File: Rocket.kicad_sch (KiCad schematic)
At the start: 6 parts, among them U1 BMP280, U2 MPU-6050, U3 ArduinoMicroSD, U4 NEO_6M, U5 FT232RL

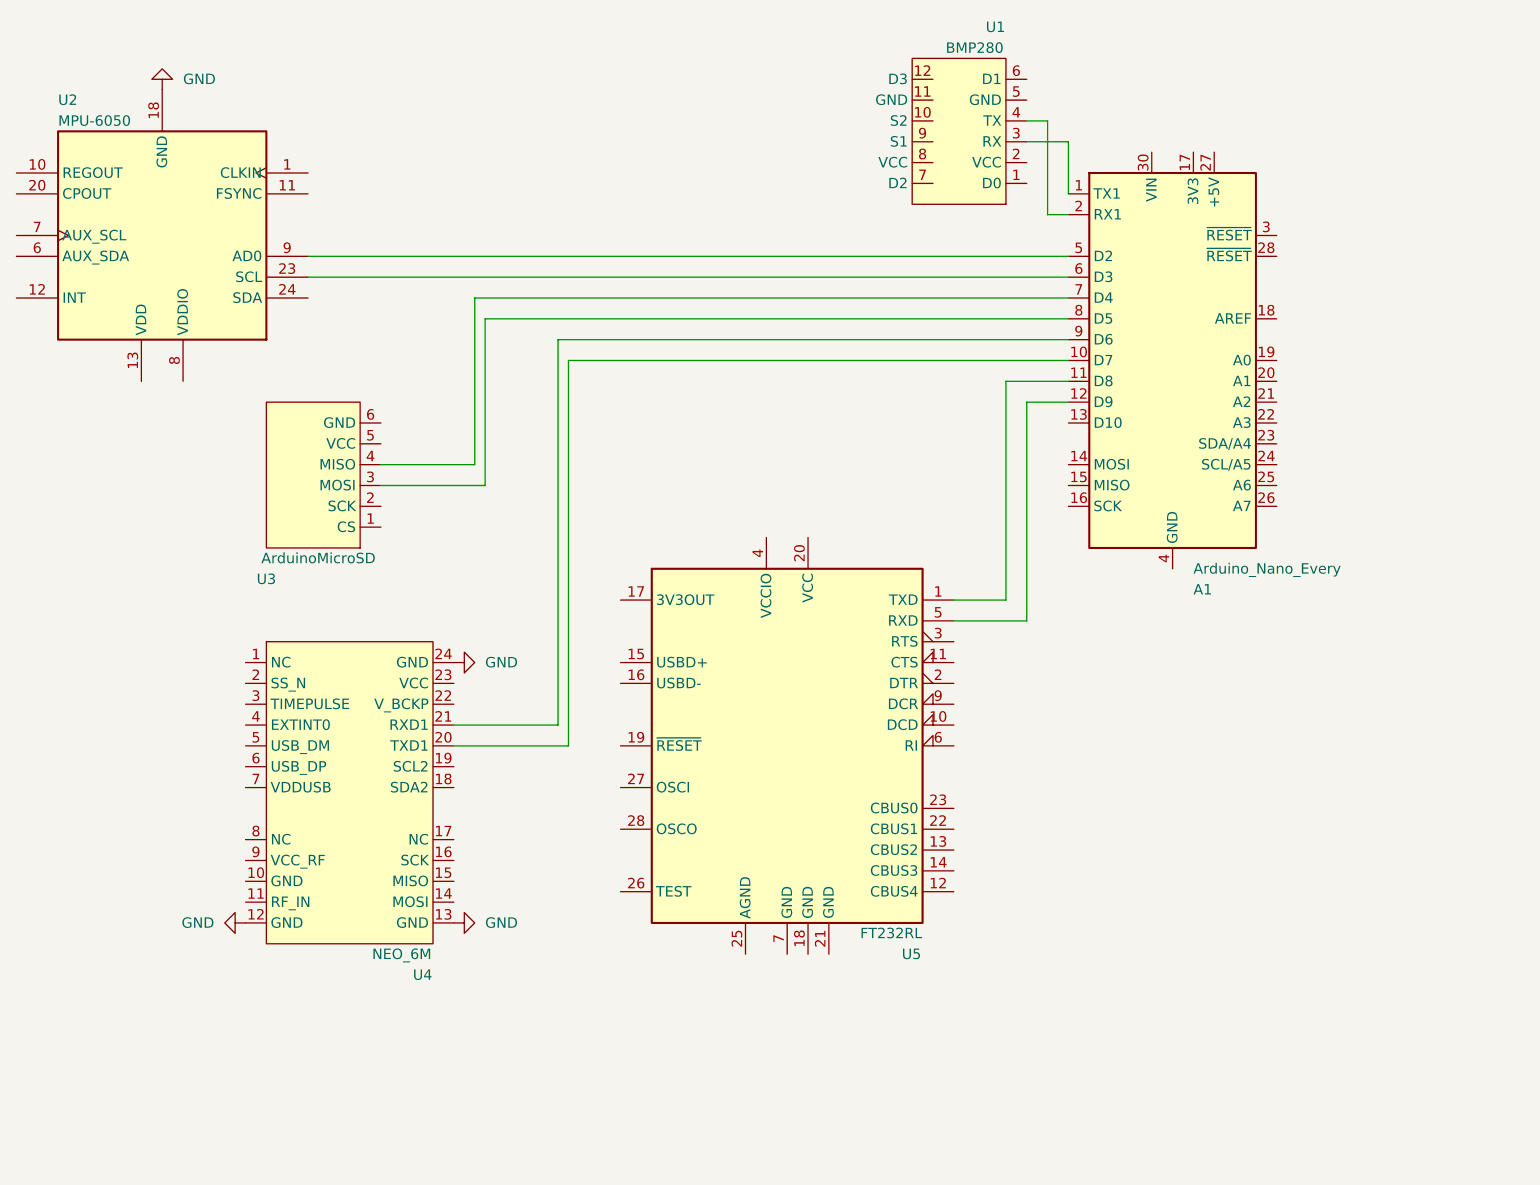
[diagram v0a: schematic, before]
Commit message: second commit: update
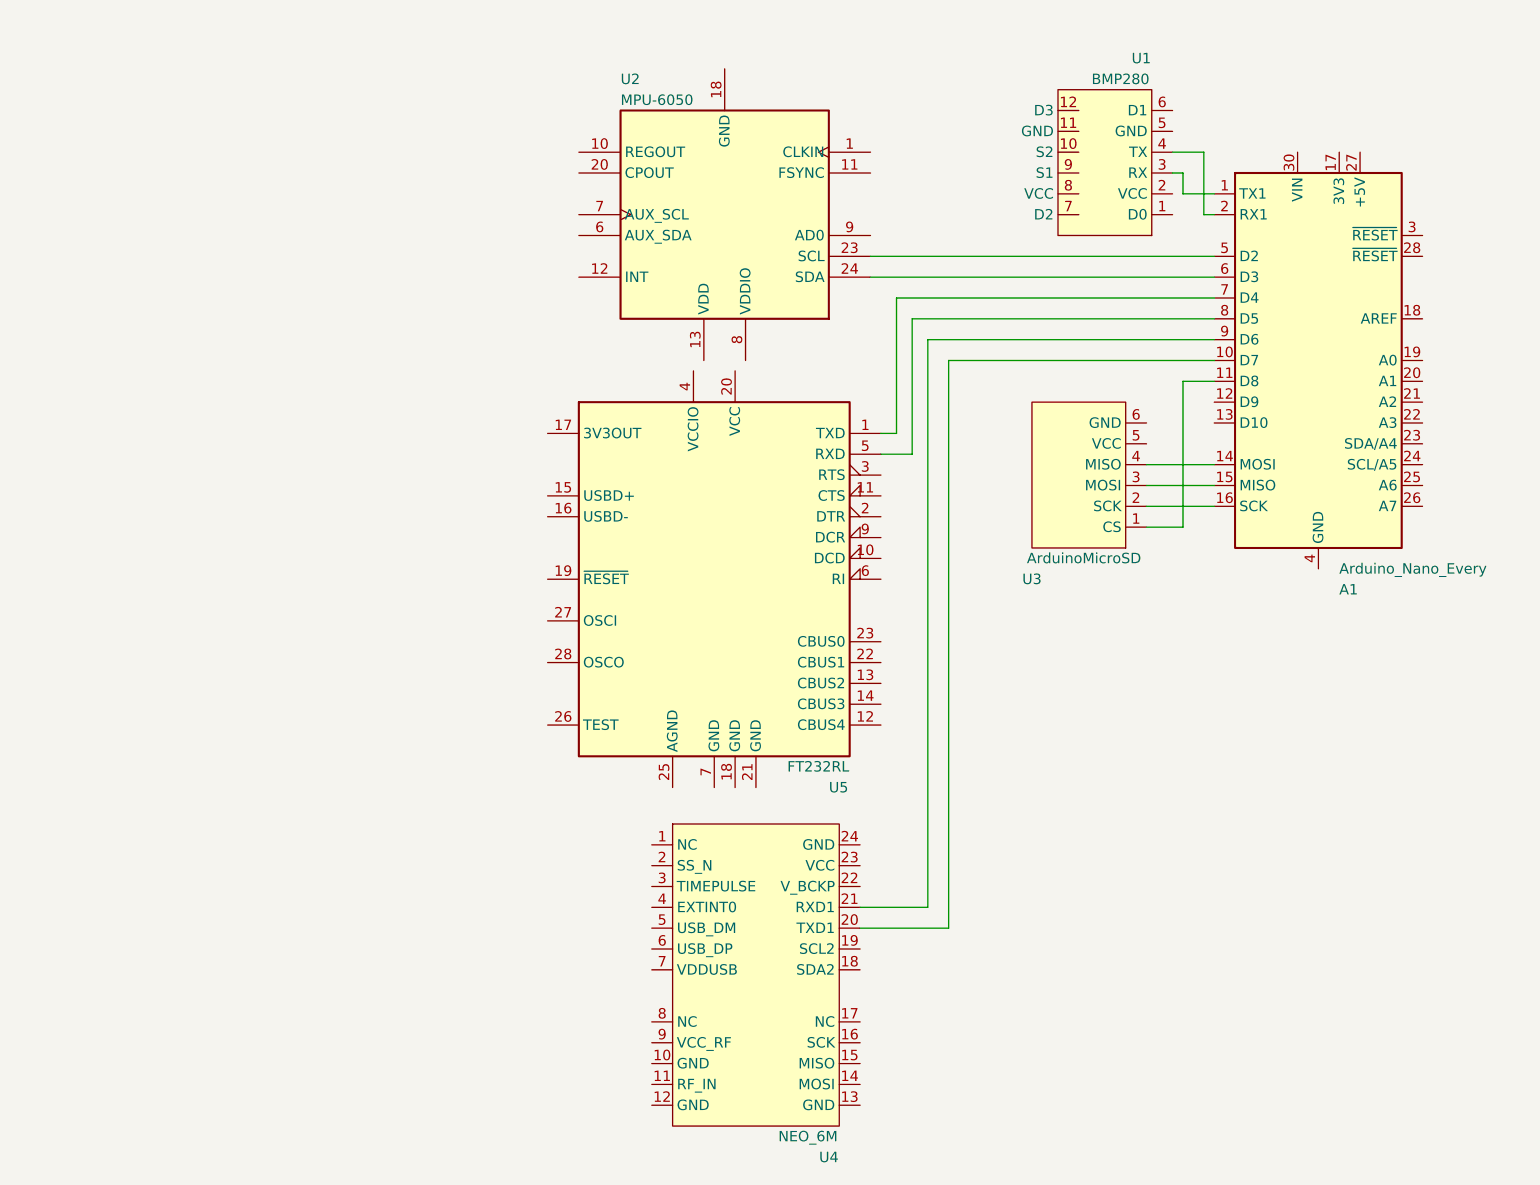
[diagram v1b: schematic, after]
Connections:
- net at U2.23 (SCL): now also A1.5 (D2); no longer A1.6 (D3)
- net at U2.24 (SDA): now also A1.6 (D3)
- net at U2.9 (AD0): no longer A1.5 (D2)
- net at U3.1 (CS): now also A1.11 (D8)
- net at U3.2 (SCK): now also A1.16 (SCK)
- net at U3.3 (MOSI): now also A1.15 (MISO); no longer A1.8 (D5)
- net at U3.4 (MISO): now also A1.14 (MOSI); no longer A1.7 (D4)
- net at U5.1 (TXD): now also A1.7 (D4); no longer A1.11 (D8)
- net at U5.5 (RXD): now also A1.8 (D5); no longer A1.12 (D9)
- removed net GND: U2.18 (GND), U4.12 (GND), U4.13 (GND), U4.24 (GND)
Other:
- moved on the sheet: A1, U1, U2, U3, U4, U5
